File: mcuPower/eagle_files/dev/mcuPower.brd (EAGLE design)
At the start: 27 x 45.1 mm, 8 parts, among them P1 CR2032, P2 CR2032, U1 PQ070XF01SZH

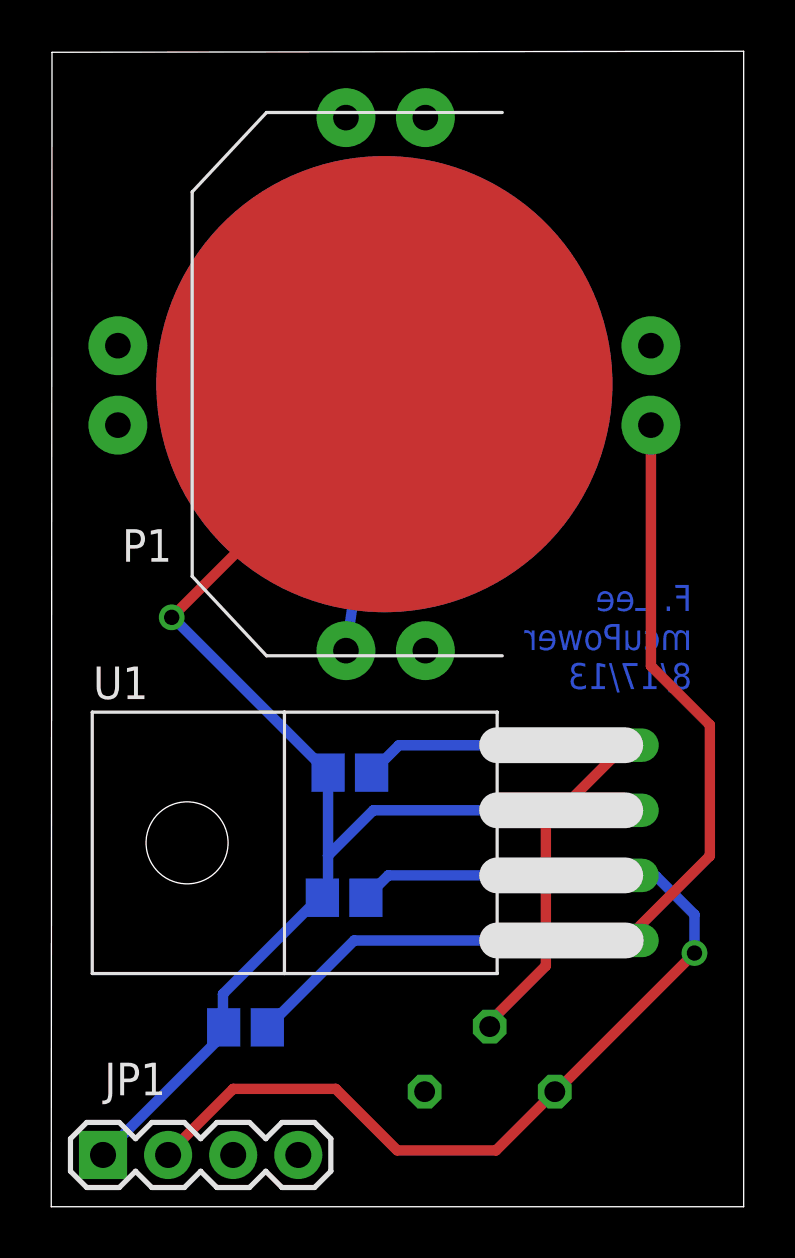
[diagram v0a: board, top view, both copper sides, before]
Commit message: most complete to date files
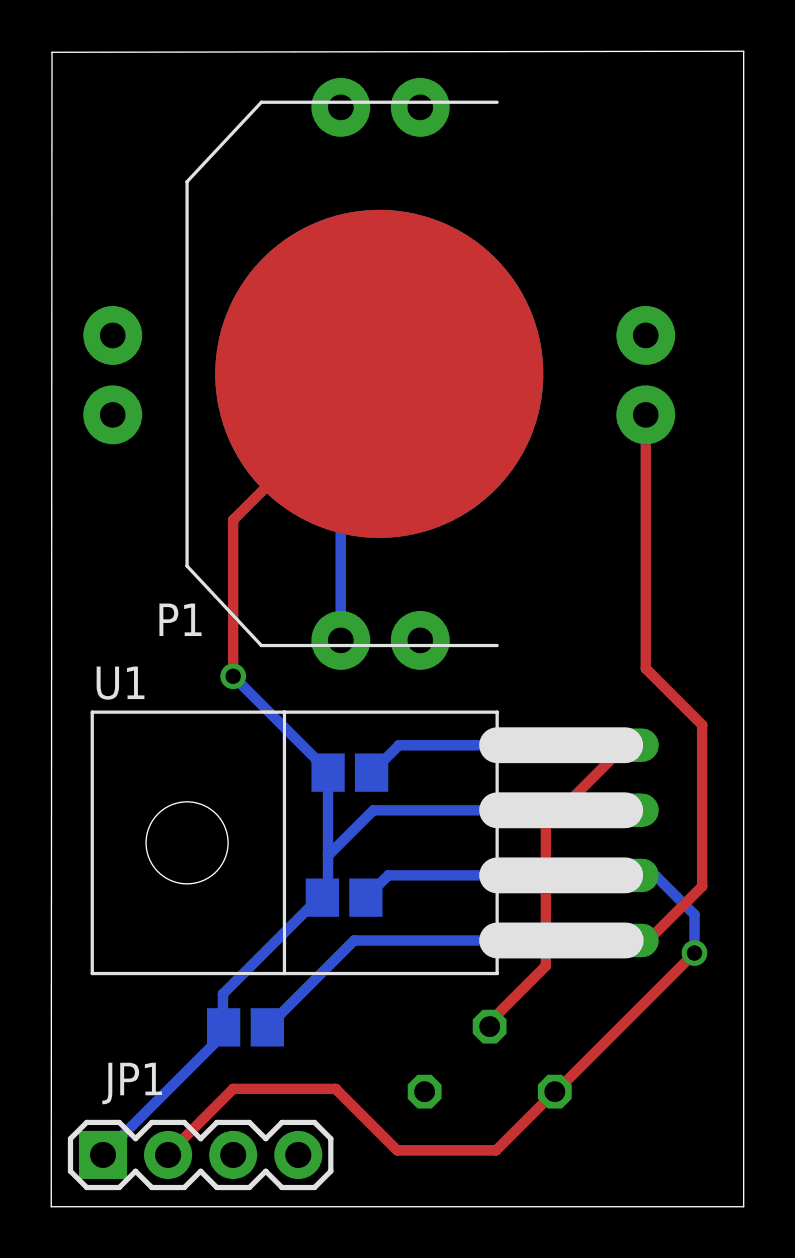
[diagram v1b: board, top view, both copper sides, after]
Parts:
- moved P1 0.45 mm to (12.8, 32.5)
- moved P2 0.45 mm to (12.8, 32.5)
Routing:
- net GND: track 52.1 -> 50.4 mm
- net VCC: track 37.8 -> 38.6 mm
- net N$1: track 10.5 -> 11.0 mm
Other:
- board text added: "F. Lee mcuPower 8/25/13"
- board text removed: "F. Lee mcuPower 8/17/13"
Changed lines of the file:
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@@
 <layer number="27" name="tValues" color="7" fill="1" visible="yes" active="yes"/>
 <layer number="28" name="bValues" color="7" fill="1" visible="yes" active="yes"/>
-<layer number="29" name="tStop" color="7" fill="3" visible="yes" active="yes"/>
-<layer number="30" name="bStop" color="7" fill="6" visible="yes" active="yes"/>
-<layer number="31" name="tCream" color="7" fill="4" visible="yes" active="yes"/>
-<layer number="32" name="bCream" color="7" fill="5" visible="yes" active="yes"/>
+<layer number="29" name="tStop" color="7" fill="3" visible="no" active="yes"/>
+<layer number="30" name="bStop" color="7" fill="6" visible="no" active="yes"/>
+<layer number="31" name="tCream" color="7" fill="4" visible="no" active="yes"/>
+<layer number="32" name="bCream" color="7" fill="5" visible="no" active="yes"/>
 <layer number="33" name="tFinish" color="6" fill="3" visible="no" active="yes"/>
 <layer number="34" name="bFinish" color="6" fill="6" visible="no" active="yes"/>
@@
 <layer number="109" name="fp9" color="7" fill="1" visible="no" active="yes"/>
 <layer number="110" name="fp0" color="7" fill="1" visible="no" active="yes"/>
-<layer number="111" name="LPC17xx" color="7" fill="1" visible="yes" active="yes"/>
-<layer number="112" name="tSilk" color="7" fill="1" visible="yes" active="yes"/>
+<layer number="111" name="LPC17xx" color="7" fill="1" visible="no" active="yes"/>
+<layer number="112" name="tSilk" color="7" fill="1" visible="no" active="yes"/>
 <layer number="116" name="Patch_BOT" color="9" fill="4" visible="yes" active="yes"/>
-<layer number="121" name="_tsilk" color="7" fill="1" visible="yes" active="yes"/>
-<layer number="122" name="_bsilk" color="7" fill="1" visible="yes" active="yes"/>
-<layer number="123" name="tTestmark" color="7" fill="1" visible="yes" active="yes"/>
-<layer number="124" name="bTestmark" color="7" fill="1" visible="yes" active="yes"/>
-<layer number="125" name="_tNames" color="7" fill="1" visible="yes" active="yes"/>
-<layer number="126" name="_bNames" color="7" fill="1" visible="yes" active="yes"/>
-<layer number="127" name="_tValues" color="7" fill="1" visible="yes" active="yes"/>
-<layer number="128" name="_bValues" color="7" fill="1" visible="yes" active="yes"/>
-<layer number="131" name="tAdjust" color="7" fill="1" visible="yes" active="yes"/>
+<layer number="121" name="_tsilk" color="7" fill="1" visible="no" active="yes"/>
+<layer number="122" name="_bsilk" color="7" fill="1" visible="no" active="yes"/>
+<layer number="123" name="tTestmark" color="7" fill="1" visible="no" active="yes"/>
+<layer number="124" name="bTestmark" color="7" fill="1" visible="no" active="yes"/>
+<layer number="125" name="_tNames" color="7" fill="1" visible="no" active="yes"/>
+<layer number="126" name="_bNames" color="7" fill="1" visible="no" active="yes"/>
+<layer number="127" name="_tValues" color="7" fill="1" visible="no" active="yes"/>
+<layer number="128" name="_bValues" color="7" fill="1" visible="no" active="yes"/>
+<layer number="131" name="tAdjust" color="7" fill="1" visible="no" active="yes"/>
 <layer number="132" name="bAdjust" color="7" fill="1" visible="no" active="yes"/>
 <layer number="144" name="Drill_legend" color="7" fill="1" visible="yes" active="yes"/>
 <layer number="150" name="Notes" color="7" fill="1" visible="no" active="yes"/>
 <layer number="151" name="HeatSink" color="7" fill="1" visible="yes" active="yes"/>
-<layer number="152" name="_bDocu" color="7" fill="1" visible="yes" active="yes"/>
+<layer number="152" name="_bDocu" color="7" fill="1" visible="no" active="yes"/>
 <layer number="153" name="FabDoc1" color="6" fill="1" visible="no" active="no"/>
 <layer number="154" name="FabDoc2" color="2" fill="1" visible="no" active="no"/>
@@
 <wire x1="27.02" y1="45.09" x2="0.03" y2="45.05" width="0" layer="20"/>
 <wire x1="0.03" y1="45.05" x2="0" y2="0" width="0" layer="20"/>
-<text x="25" y="20.2" size="1.016" layer="16" rot="MR0">F. Lee
+<text x="25.3" y="20.5" size="1.016" layer="22" rot="MR0">F. Lee
 mcuPower
-8/17/13</text>
+8/25/13</text>
 </plain>
 <attributes>
@@
 <attribute name="NAME" x="3.78" y="21.08" size="1.27" layer="25" rot="R180"/>
 </element>
-<element name="P1" library="freddyLibr" package="CR2032/2025" value="CR2032" x="13" y="32.1" smashed="yes" rot="R90">
-<attribute name="NAME" x="4.71" y="26.44" size="1.27" layer="25" rot="R180"/>
-</element>
-<element name="P2" library="freddyLibr" package="CR2032/2025" value="CR2032" x="13" y="32.1" smashed="yes" rot="MR0">
-<attribute name="NAME" x="25.41" y="37.46" size="1.27" layer="26" rot="MR0"/>
+<element name="P1" library="freddyLibr" package="CR2032/2025" value="CR2032" x="12.8" y="32.5" smashed="yes" rot="R90">
+<attribute name="NAME" x="6.01" y="23.54" size="1.27" layer="25" rot="R180"/>
+</element>
+<element name="P2" library="freddyLibr" package="CR2032/2025" value="CR2032" x="12.8" y="32.5" smashed="yes" rot="MR0">
+<attribute name="NAME" x="21.01" y="41.16" size="1.27" layer="26" rot="MR0"/>
 </element>
 </elements>
@@
 <contactref element="C1" pad="1"/>
 <contactref element="U1" pad="VIN"/>
-<contactref element="P2" pad="VCC_2"/>
 <wire x1="22.4" y1="10.39" x2="11.82" y2="10.39" width="0.4064" layer="16"/>
 <wire x1="11.82" y1="10.39" x2="8.43" y2="7" width="0.4064" layer="16"/>
-<wire x1="23.4" y1="30.5" x2="23.4" y2="21.1" width="0.4064" layer="1"/>
-<wire x1="23.4" y1="21.1" x2="25.7" y2="18.8" width="0.4064" layer="1"/>
-<wire x1="25.7" y1="18.8" x2="25.7" y2="13.69" width="0.4064" layer="1"/>
-<wire x1="25.7" y1="13.69" x2="22.4" y2="10.39" width="0.4064" layer="1"/>
+<contactref element="P2" pad="VCC_2"/>
+<wire x1="23.2" y1="30.9" x2="23.2" y2="21" width="0.4064" layer="1"/>
+<wire x1="23.2" y1="21" x2="25.4" y2="18.8" width="0.4064" layer="1"/>
+<wire x1="25.4" y1="18.8" x2="25.4" y2="12.5" width="0.4064" layer="1"/>
+<wire x1="25.4" y1="12.5" x2="23.3" y2="10.4" width="0.4064" layer="1"/>
+<wire x1="23.3" y1="10.4" x2="22.41" y2="10.4" width="0.4064" layer="1"/>
+<wire x1="22.41" y1="10.4" x2="22.4" y2="10.39" width="0.4064" layer="1"/>
 </signal>
 <signal name="GND">
@@
 <contactref element="JP1" pad="1"/>
 <contactref element="U1" pad="GND"/>
-<contactref element="P1" pad="GND"/>
-<wire x1="13" y1="32.1" x2="13" y2="31.3" width="0.4064" layer="1"/>
-<wire x1="13" y1="31.3" x2="4.7" y2="23" width="0.4064" layer="1"/>
-<via x="4.7" y="23" extent="1-16" drill="0.6"/>
-<wire x1="4.7" y1="23" x2="4.74" y2="23" width="0.4064" layer="16"/>
-<wire x1="4.74" y1="23" x2="10.8" y2="16.94" width="0.4064" layer="16"/>
 <wire x1="10.8" y1="16.94" x2="10.8" y2="13.7" width="0.4064" layer="16"/>
 <wire x1="10.8" y1="13.7" x2="10.8" y2="12.28" width="0.4064" layer="16"/>
@@
 <wire x1="22.4" y1="15.47" x2="12.57" y2="15.47" width="0.4064" layer="16"/>
 <wire x1="12.57" y1="15.47" x2="10.8" y2="13.7" width="0.4064" layer="16"/>
+<contactref element="P1" pad="GND"/>
+<wire x1="10.8" y1="16.94" x2="10.8" y2="17" width="0.4064" layer="16"/>
+<wire x1="10.8" y1="17" x2="7.1" y2="20.7" width="0.4064" layer="16"/>
+<via x="7.1" y="20.7" extent="1-16" drill="0.6"/>
+<wire x1="7.1" y1="20.7" x2="7.1" y2="26.8" width="0.4064" layer="1"/>
+<wire x1="7.1" y1="26.8" x2="12.8" y2="32.5" width="0.4064" layer="1"/>
 </signal>
 <signal name="N$2">
@@
 <contactref element="JP1" pad="4"/>
 </signal>
+<signal name="N$3">
+</signal>
 <signal name="N$1">
 <contactref element="P1" pad="VCC_1"/>
 <contactref element="P2" pad="GND"/>
-<wire x1="11.5" y1="21.7" x2="12.8" y2="30.6" width="0.4064" layer="16"/>
-<wire x1="12.8" y1="30.6" x2="13" y2="32.1" width="0.4064" layer="16"/>
-</signal>
-<signal name="N$3">
+<wire x1="11.3" y1="22.1" x2="11.3" y2="31" width="0.4064" layer="16"/>
+<wire x1="11.3" y1="31" x2="12.8" y2="32.5" width="0.4064" layer="16"/>
 </signal>
 </signals>
